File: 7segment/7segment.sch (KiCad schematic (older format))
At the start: 33 parts, among them J1 Barrel_Jack, J2 Conn_Segments, J3 Conn_Segments, J4 Conn_Segments, J5 DB9_Male, SW1 SW_Push, SW2 SW_Push, U1 ULN2803A, U2 2981, U3 2981, U4 L7809, U5 74HC595, U6 74HC595, U7 4017, U8 StepUp, U9 Max3232Board

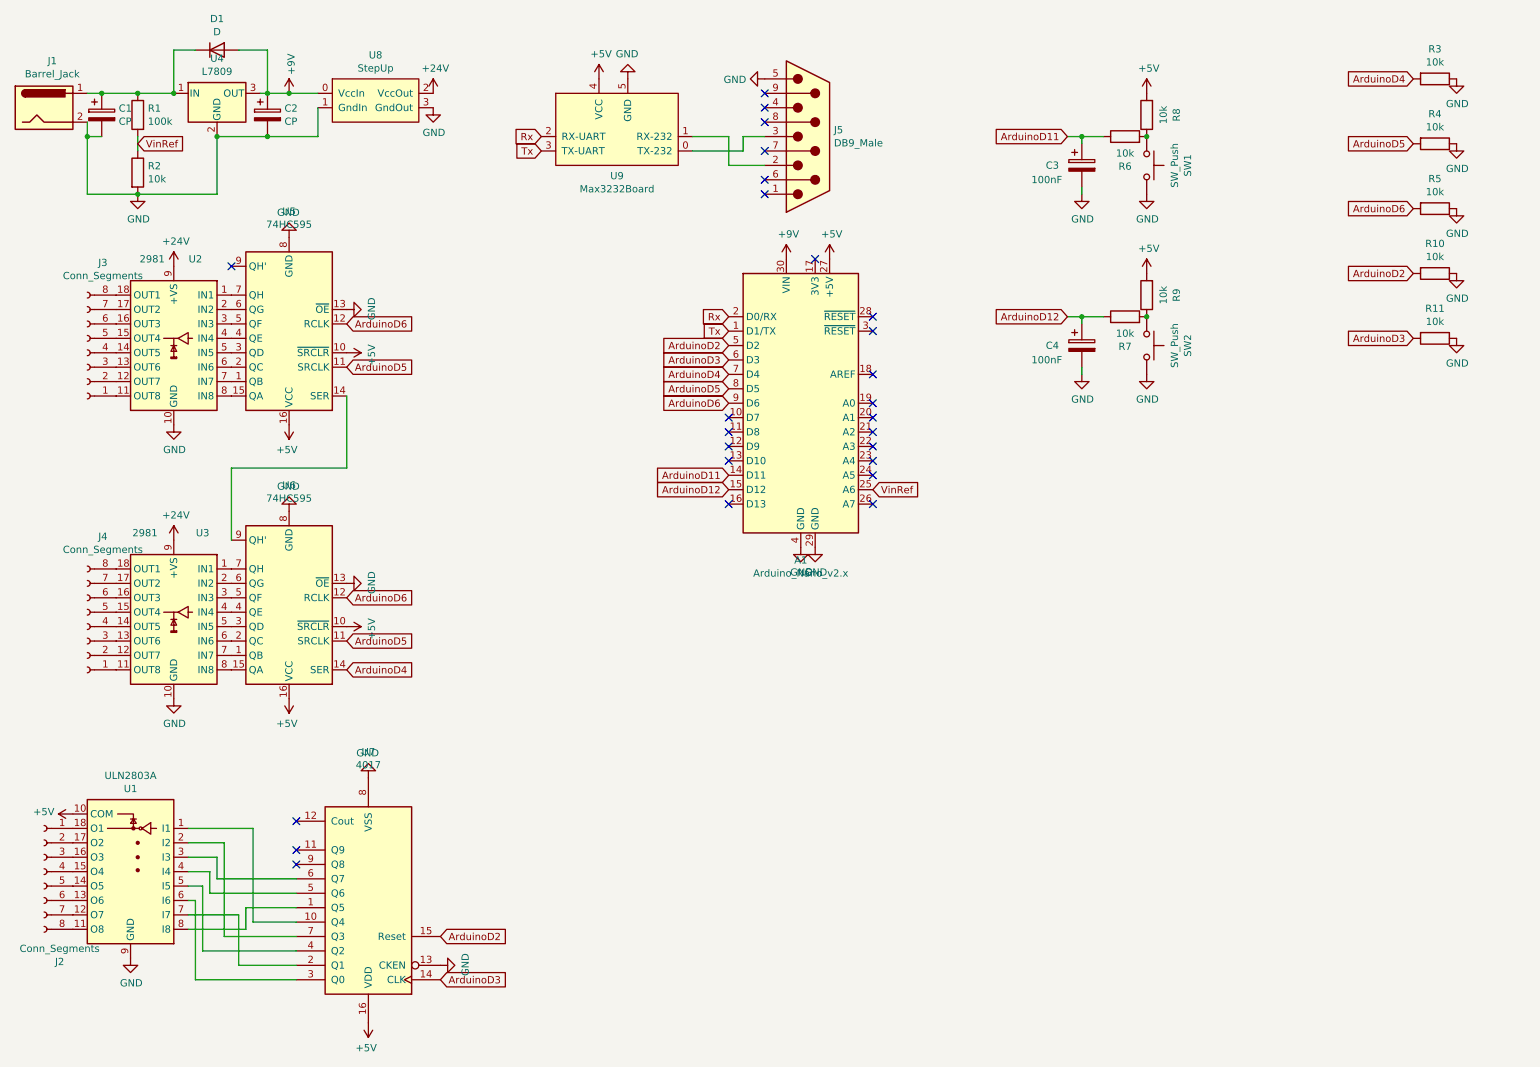
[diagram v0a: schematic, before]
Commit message: KiCad: Platinen Version 1
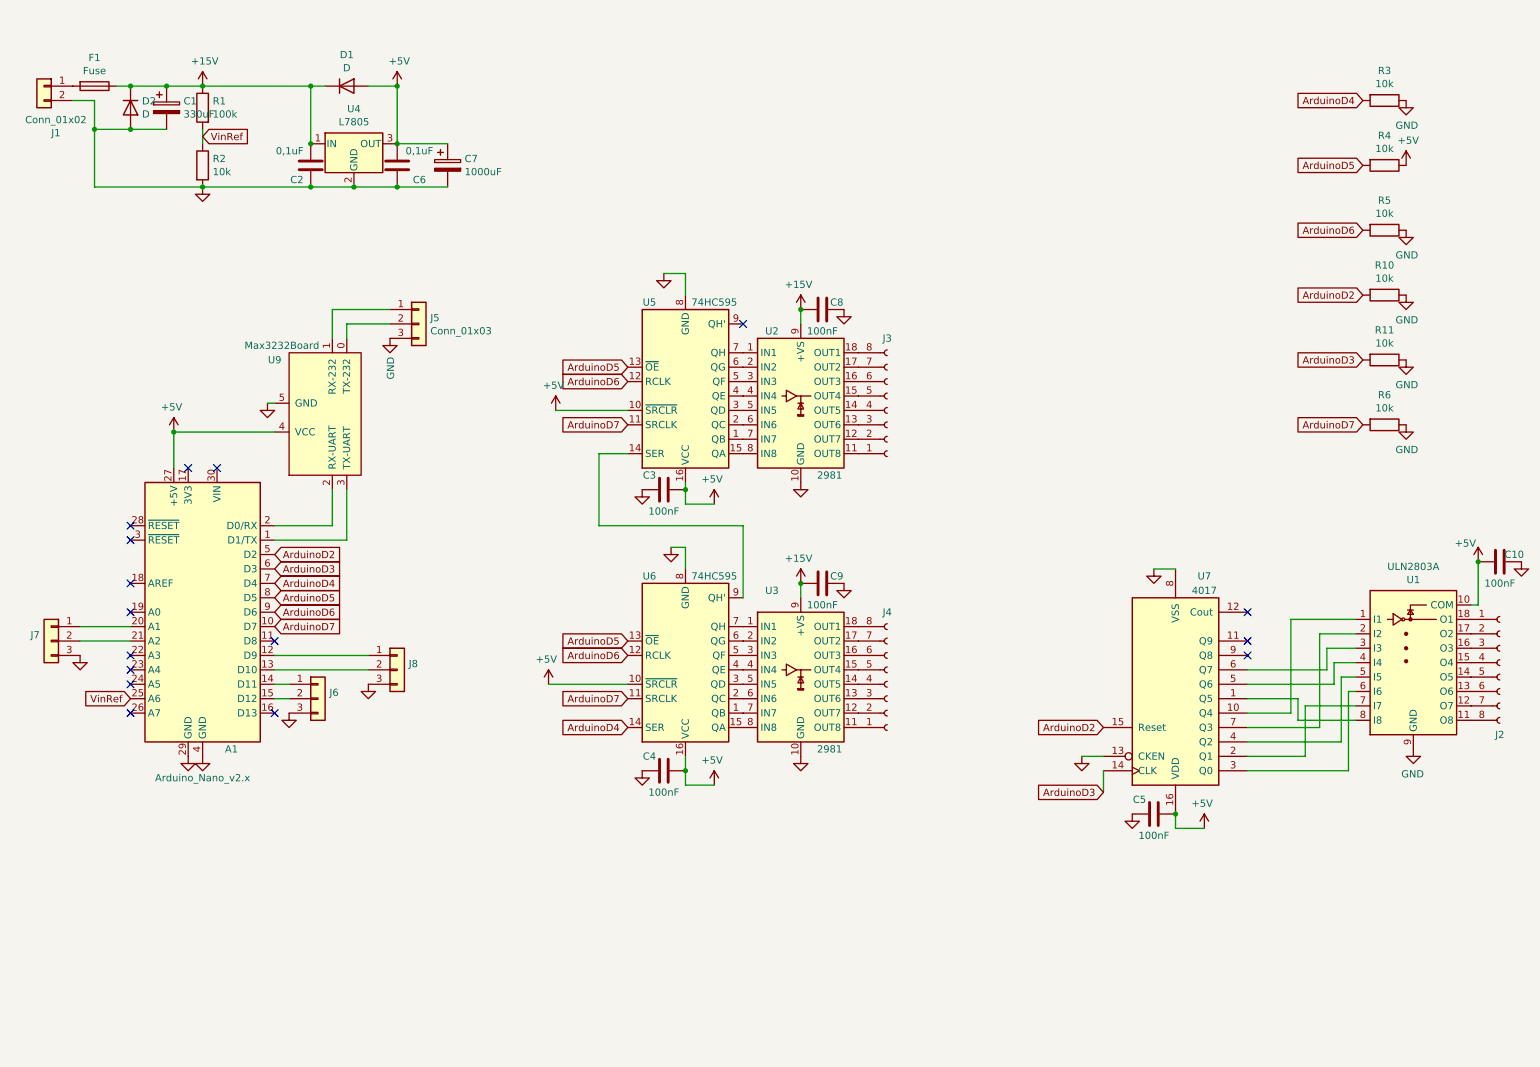
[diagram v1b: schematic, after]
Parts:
- removed C2: CP, Capacitor_THT:CP_Radial_D5.0mm_P2.50mm, symbol Device:CP
- removed C3, C4: 100nF, Capacitor_THT:CP_Radial_D5.0mm_P2.50mm, symbol Device:CP
- removed J1: Barrel_Jack, Connector_PinHeader_2.54mm:PinHeader_1x02_P2.54mm_Vertical, symbol Connector:Barrel_Jack
- removed J5: DB9_Male, Connector_Dsub:DSUB-9_Male_Vertical_P2.77x2.84mm, symbol Connector:DB9_Male
- removed R7: 10k, Resistor_THT:R_Axial_DIN0309_L9.0mm_D3.2mm_P12.70mm_Horizontal, symbol Device:R
- removed R8, R9: 10k, Resistor_THT:R_Axial_DIN0204_L3.6mm_D1.6mm_P7.62mm_Horizontal, symbol Device:R
- removed SW1, SW2: SW_Push, Button_Switch_THT:SW_PUSH_6mm_H7.3mm, symbol Switch:SW_Push
- removed U4: L7809, Connector_PinSocket_2.54mm:PinSocket_1x03_P2.54mm_Vertical, symbol Regulator_Linear:L7809
- removed U8: StepUp, 7segment:StepUp, symbol New_Library:StepUp
- added C10, C3, C4, C5, C8, C9: 100nF, Capacitor_THT:C_Disc_D5.0mm_W2.5mm_P2.50mm, symbol Device:C
- added C2, C6: 0,1uF, Capacitor_THT:C_Disc_D3.4mm_W2.1mm_P2.50mm, symbol Device:C
- added C7: 1000uF, Capacitor_THT:CP_Radial_D10.0mm_P5.00mm, symbol Device:CP
- added D2: D, Diode_THT:D_A-405_P7.62mm_Horizontal, symbol Device:D
- added F1: Fuse, myself:Fuse, symbol Device:Fuse
- added J1: Conn_01x02, myself:Connector 2xPin, symbol Connector_Generic:Conn_01x02
- added J5, J6, J7, J8: Conn_01x03, myself:Connector 3xPin, symbol Connector_Generic:Conn_01x03
- added U4: L7805, L7805CV:TO255P1040X460X1968-3, symbol Regulator_Linear:L7805
- C1: value CP -> 330uF; footprint Capacitor_THT:CP_Radial_D5.0mm_P2.50mm -> Capacitor_THT:CP_Radial_D10.0mm_P5.00mm
- D1: footprint Diode_THT:D_A-405_P5.08mm_Vertical_KathodeUp -> Diode_THT:D_A-405_P10.16mm_Horizontal
- R1, R10, R3: footprint Resistor_THT:R_Axial_DIN0204_L3.6mm_D1.6mm_P7.62mm_Horizontal -> myself:Resistor, L6mm,4holes
- R11, R4: footprint Resistor_THT:R_Axial_DIN0204_L3.6mm_D1.6mm_P7.62mm_Horizontal -> myself:Resistor, L6mm,5holes
- R2, R6: footprint Resistor_THT:R_Axial_DIN0207_L6.3mm_D2.5mm_P10.16mm_Horizontal -> myself:Resistor, L6mm,5holes
- R5: footprint Resistor_THT:R_Axial_DIN0207_L6.3mm_D2.5mm_P10.16mm_Horizontal -> myself:Resistor, L6mm,6holes
- U1: footprint Package_DIP:DIP-18_W7.62mm -> Package_DIP:DIP-18_W7.62mm_LongPads
- U5, U6, U7: footprint Package_DIP:DIP-16_W7.62mm -> Package_DIP:DIP-16_W7.62mm_LongPads
- U9: footprint 7segment:MAX232 -> myself:MAX232
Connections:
- net +24V is gone; now on net +15V: U2.9 (+VS), U3.9 (+VS)
- net +5V: now also D1.2 (A), R4.1, C10.1, C3.2, C4.2, C5.2, C6.2, C7.1, U4.3 (OUT)
- net ArduinoD5: now also U5.13 (~OE), U6.13 (~OE); no longer U5.11 (SRCLK), U6.11 (SRCLK)
- net GND: now also R6.1, C10.2, C2.1, C3.1, C4.1, C5.1, C6.1, C7.2, C8.2, C9.2, D2.2 (A), J1.2 (Pin_2), J5.3 (Pin_3), J6.3 (Pin_3), J7.3 (Pin_3), J8.3 (Pin_3), U4.2 (GND); no longer R4.1, U5.13 (~OE), U6.13 (~OE)
- net ArduinoD7: now reaches A1.10 (D7)
- net ArduinoD7: now also R6.2, U5.11 (SRCLK), U6.11 (SRCLK)
- net at A1.12 (D9): now also J8.1 (Pin_1)
- net at A1.13 (D10): now also J8.2 (Pin_2)
- net at A1.20 (A1): now also J7.1 (Pin_1)
- net at A1.21 (A2): now also J7.2 (Pin_2)
- net at U9.0 (TX-232): now also J5.2 (Pin_2)
- net at U9.1 (RX-232): now also J5.1 (Pin_1)
- net +15V: now reaches C1.1, D1.1 (K), R1.1
- net +15V: now also C2.2, C8.1, C9.1, D2.1 (K), F1.1, U4.1 (IN)
- net +9V: no longer names the net of A1.30 (VIN)
- net +9V: no longer D1.2 (A)
- net ArduinoD11: no longer names the net of A1.14 (D11)
- net ArduinoD11: now also J6.1 (Pin_1); no longer R6.1
- net ArduinoD12: no longer names the net of A1.15 (D12)
- net ArduinoD12: now also J6.2 (Pin_2)
- net Rx: no longer names the net of A1.2 (D0/RX), U9.2 (RX-UART)
- net Tx: no longer names the net of A1.1 (D1/TX), U9.3 (TX-UART)
- new net: F1.2, J1.1 (Pin_1)
- no-connect marks 26 -> 16
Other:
- moved on the sheet: A1, C1, D1, J2, J3, J4, R1, R10, R11, R2, R3, R4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
